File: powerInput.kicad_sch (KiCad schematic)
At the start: 12 parts, among them IC11 LM74700QDBVRQ1, IC12 LM74700QDBVRQ1, IC13 LM74700QDBVRQ1, IC18 INA260AIPWR, IC8 INA260AIPWR, IC9 INA260AIPWR, Q4 BSZ067N06LS3_G, Q5 BSZ067N06LS3_G, Q6 BSZ067N06LS3_G

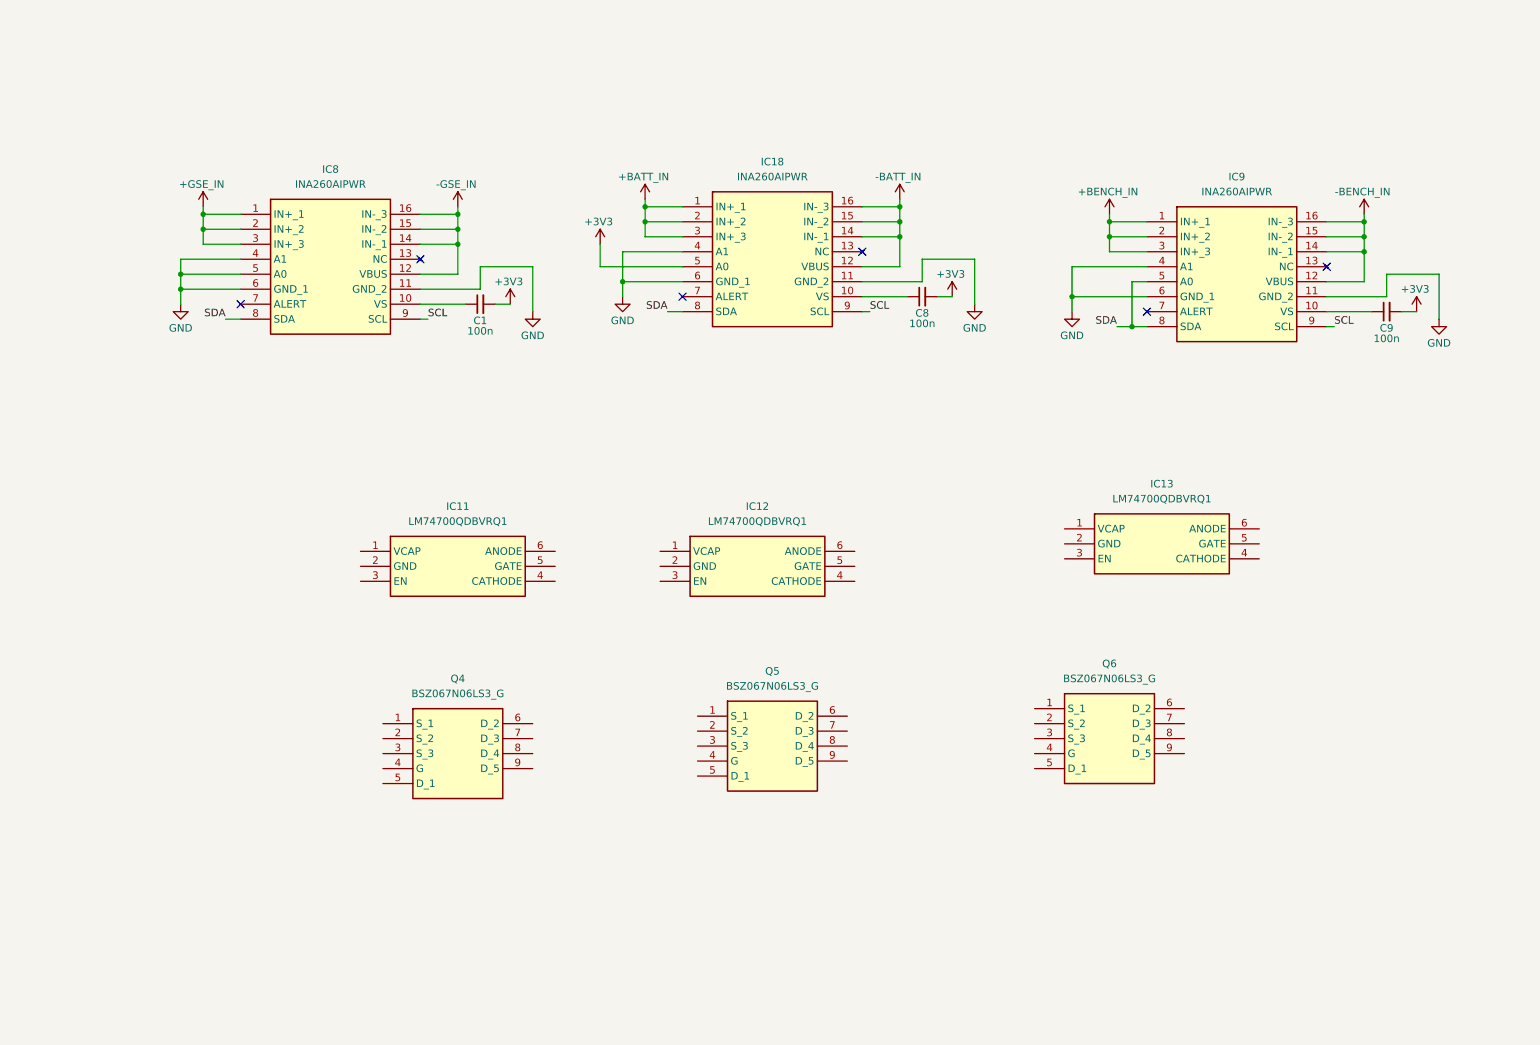
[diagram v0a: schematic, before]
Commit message: Test commit
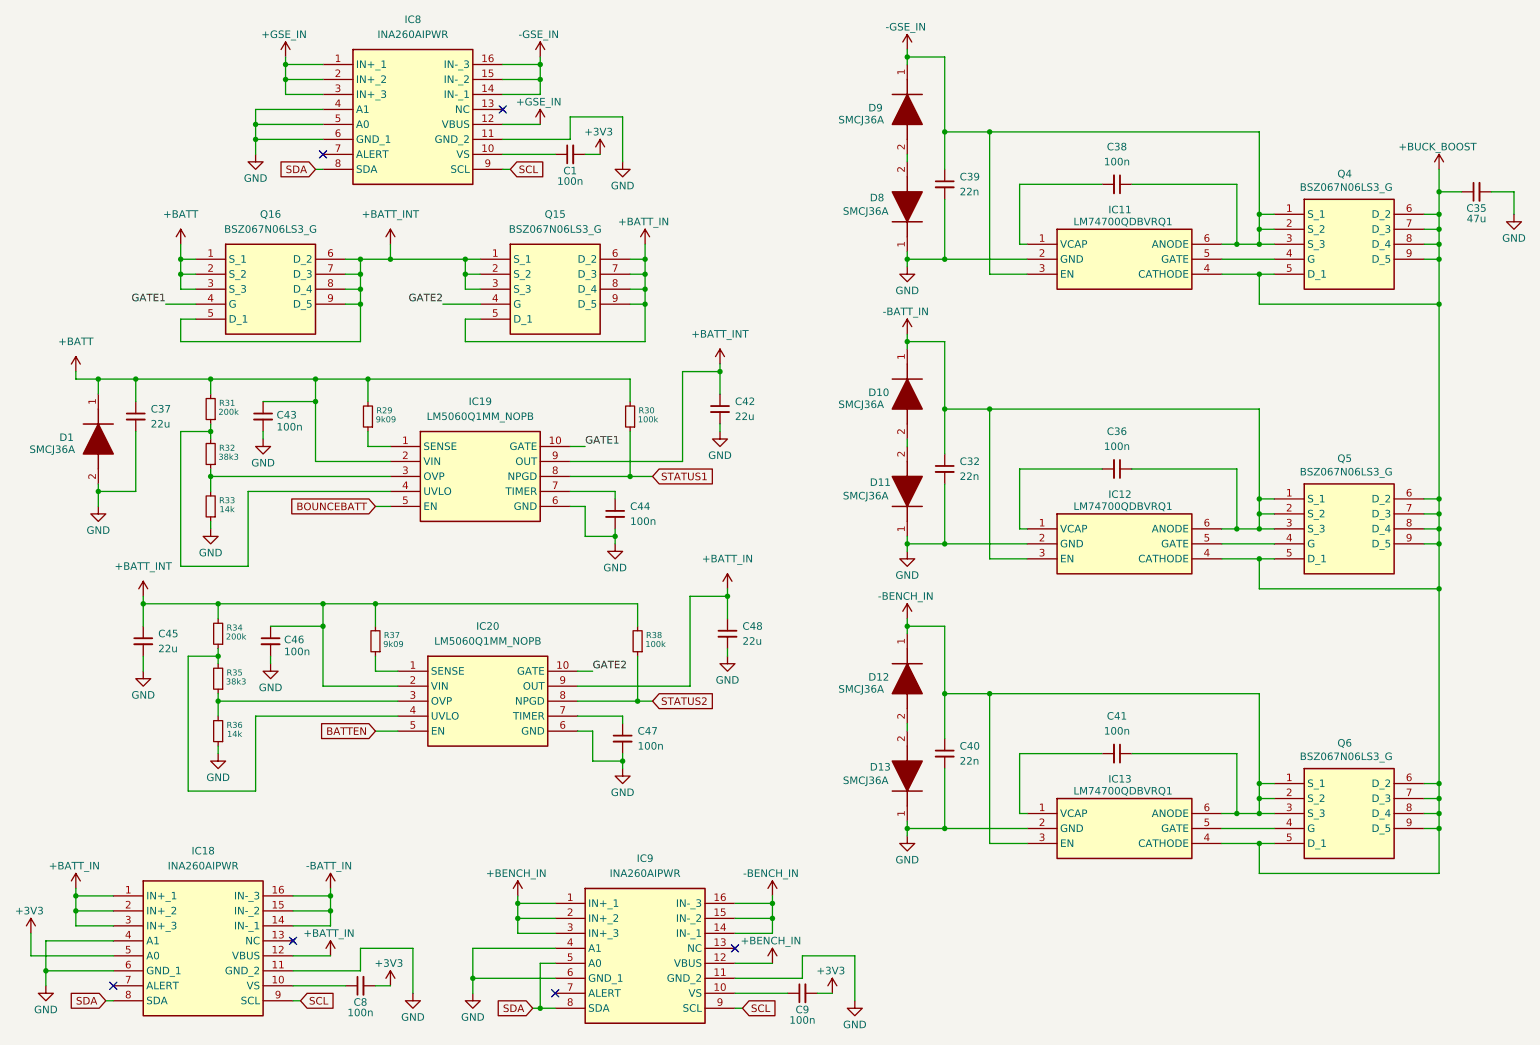
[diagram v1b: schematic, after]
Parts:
- added C32, C39, C40: 22n, symbol Device:C_Small
- added C35: 47u, symbol Device:C_Small
- added C36, C38, C41, C43, C44, C46, C47: 100n, symbol Device:C_Small
- added C37, C42, C45, C48: 22u, symbol Device:C_Small
- added D1, D10, D11, D12, D13, D8, D9: SMCJ36A, DIOM8059X256N, symbol HEDGE2:SMCJ36A
- added IC19, IC20: LM5060Q1MM_NOPB, SOP50P490X110-10N, symbol HEDGE2:LM5060Q1MM_NOPB
- added Q15, Q16: BSZ067N06LS3_G, BSZ067N06LS3G, symbol HEDGE2:BSZ067N06LS3_G
- added R29, R37: 9k09, symbol Device:R_Small
- added R30, R38: 100k, symbol Device:R_Small
- added R31, R34: 200k, symbol Device:R_Small
- added R32, R35: 38k3, symbol Device:R_Small
- added R33, R36: 14k, symbol Device:R_Small
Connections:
- net +BATT_IN: now also IC18.12 (VBUS), C48.1, IC20.9 (OUT), Q15.5 (D_1), Q15.6 (D_2), Q15.7 (D_3), Q15.8 (D_4), Q15.9 (D_5)
- net +BENCH_IN: now also IC9.12 (VBUS)
- net +GSE_IN: now also IC8.12 (VBUS)
- net -BATT_IN: now also IC12.3 (EN), IC12.6 (ANODE), Q5.1 (S_1), Q5.2 (S_2), Q5.3 (S_3), C32.1, C36.1, D10.1 (K); no longer IC18.12 (VBUS)
- net -BENCH_IN: now also IC13.3 (EN), IC13.6 (ANODE), Q6.1 (S_1), Q6.2 (S_2), Q6.3 (S_3), C40.1, C41.1, D12.1 (K); no longer IC9.12 (VBUS)
- net -GSE_IN: now also IC11.3 (EN), IC11.6 (ANODE), Q4.1 (S_1), Q4.2 (S_2), Q4.3 (S_3), C38.1, C39.1, D9.1 (K); no longer IC8.12 (VBUS)
- net GND: now also IC11.2 (GND), IC12.2 (GND), IC13.2 (GND), C32.2, C35.2, C37.2, C39.2, C40.2, C42.2, C43.2, C44.2, C45.2, C46.2, C47.2, C48.2, D1.2 (A), D11.1 (K), D13.1 (K), D8.1 (K), IC19.6 (GND), IC20.6 (GND), R33.1, R36.1
- net at IC11.1 (VCAP): now also C38.2
- net +BUCK_BOOST: now reaches IC11.4 (CATHODE)
- net +BUCK_BOOST: now also IC12.4 (CATHODE), IC13.4 (CATHODE), Q4.5 (D_1), Q4.6 (D_2), Q4.7 (D_3), Q4.8 (D_4), Q4.9 (D_5), Q5.5 (D_1), Q5.6 (D_2), Q5.7 (D_3), Q5.8 (D_4), Q5.9 (D_5), Q6.5 (D_1), Q6.6 (D_2), Q6.7 (D_3), Q6.8 (D_4), Q6.9 (D_5), C35.1
- net at IC11.5 (GATE): now also Q4.4 (G)
- net at Q5.4 (G): now also IC12.5 (GATE)
- net at IC12.1 (VCAP): now also C36.2
- net at Q6.4 (G): now also IC13.5 (GATE)
- net at IC13.1 (VCAP): now also C41.2
- new net: IC19.1 (SENSE), R29.1
- new net: D8.2 (A), D9.2 (A)
- new net: D12.2 (A), D13.2 (A)
- new net: IC20.3 (OVP), R35.1, R36.2
- new net: IC20.4 (UVLO), R34.1, R35.2
- new net: C47.1, IC20.7 (TIMER)
- new net: IC19.3 (OVP), R32.1, R33.2
- new net: IC19.4 (UVLO), R31.1, R32.2
- new net: C44.1, IC19.7 (TIMER)
- new net: IC20.1 (SENSE), R37.1
- new net: D10.2 (A), D11.2 (A)
- new net +BATT: C37.1, C43.1, D1.1 (K), IC19.2 (VIN), Q16.1 (S_1), Q16.2 (S_2), Q16.3 (S_3), R29.2, R30.2, R31.2
- new net +BATT_INT: C42.1, C45.1, C46.1, IC19.9 (OUT), IC20.2 (VIN), Q15.1 (S_1), Q15.2 (S_2), Q15.3 (S_3), Q16.5 (D_1), Q16.6 (D_2), Q16.7 (D_3), Q16.8 (D_4), Q16.9 (D_5), R34.2, R37.2, R38.2
- new net BATTEN: IC20.5 (EN)
- new net BOUNCEBATT: IC19.5 (EN)
- new net GATE1: IC19.10 (GATE), Q16.4 (G)
- new net GATE2: IC20.10 (GATE), Q15.4 (G)
- new net STATUS1: IC19.8 (NPGD), R30.1
- new net STATUS2: IC20.8 (NPGD), R38.1
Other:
- moved on the sheet: C1, C8, C9, IC11, IC18, IC8, IC9, Q4
